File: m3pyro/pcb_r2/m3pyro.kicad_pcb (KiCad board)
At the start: 2 copper layers, 39 x 39 mm, 67 parts, among them IC1 STM32F405RxTx, IC2 TPS62130, IC3 MCP2562, IC4 TPS62150, J1 WEST TOP, J2 WEST BOT, J3 EAST TOP, J4 EAST BOT, Q1 Si5515CDC, Q2 Si5515CDC, Q3 Si5515CDC, Q4 Si5515CDC, Q5 Si5515CDC, Q6 Si5515CDC, Q7 Si5515CDC, Q8 Si5515CDC, Y1 26M

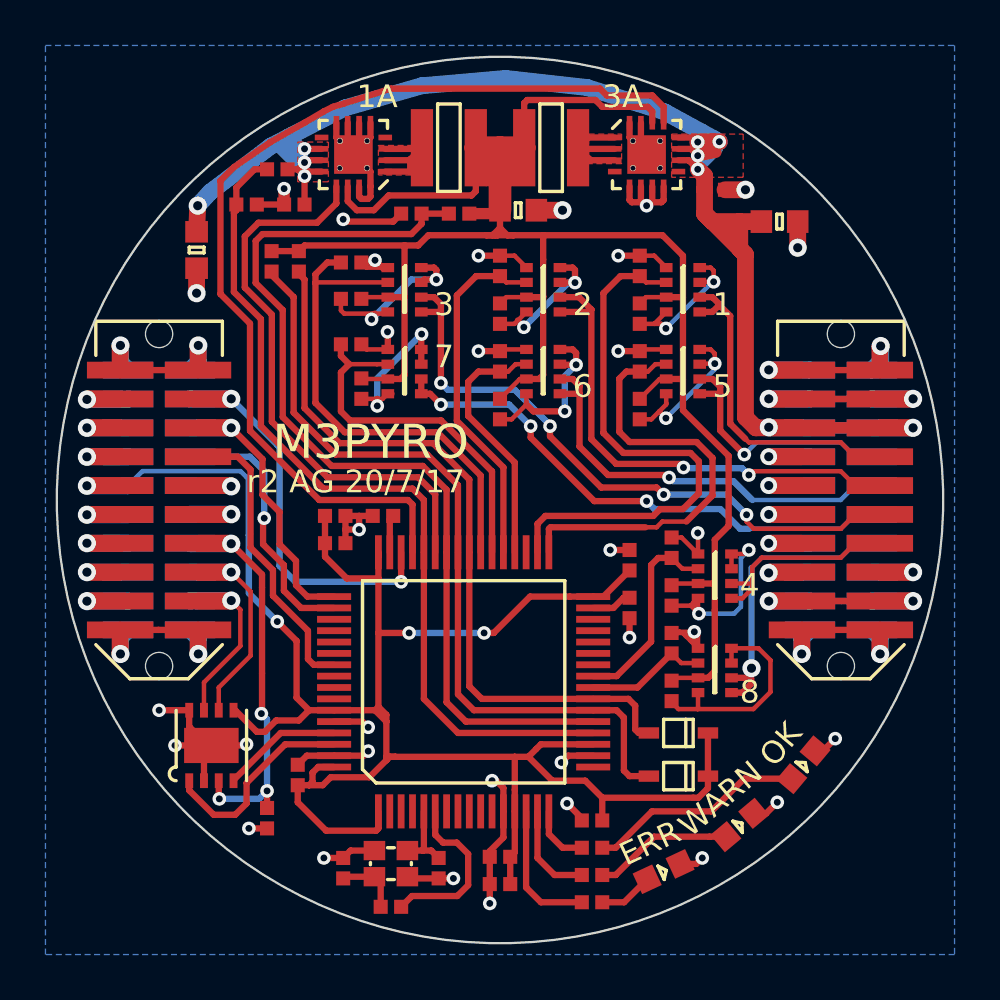
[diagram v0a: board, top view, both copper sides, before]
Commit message: slight further tidyup of myp3yro
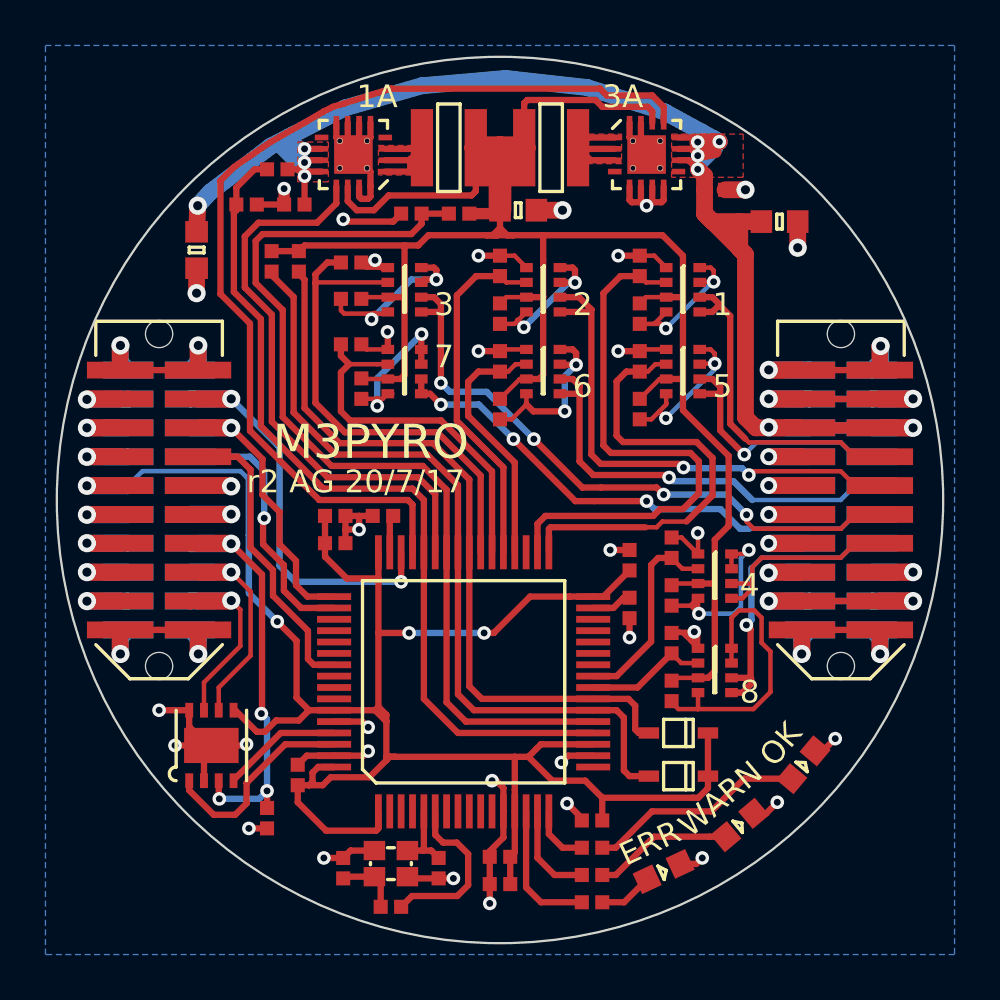
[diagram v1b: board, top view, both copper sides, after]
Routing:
- net Net-(Q8-Pad4): track 9.62 -> 12.7 mm
